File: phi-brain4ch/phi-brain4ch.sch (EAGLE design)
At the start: 65 parts, among them IC1 STM32F427VGT6, IC2 6N138S-TA1, IC3 AT45DB161D-SU, U1 LM1117MPX-3.3/NOPB or AP2114H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, U2 PRTR5V0U2X, X2 04-JST-B4B-XH-A, X3 04-JST-B4B-XH-A, Y1 8MHz

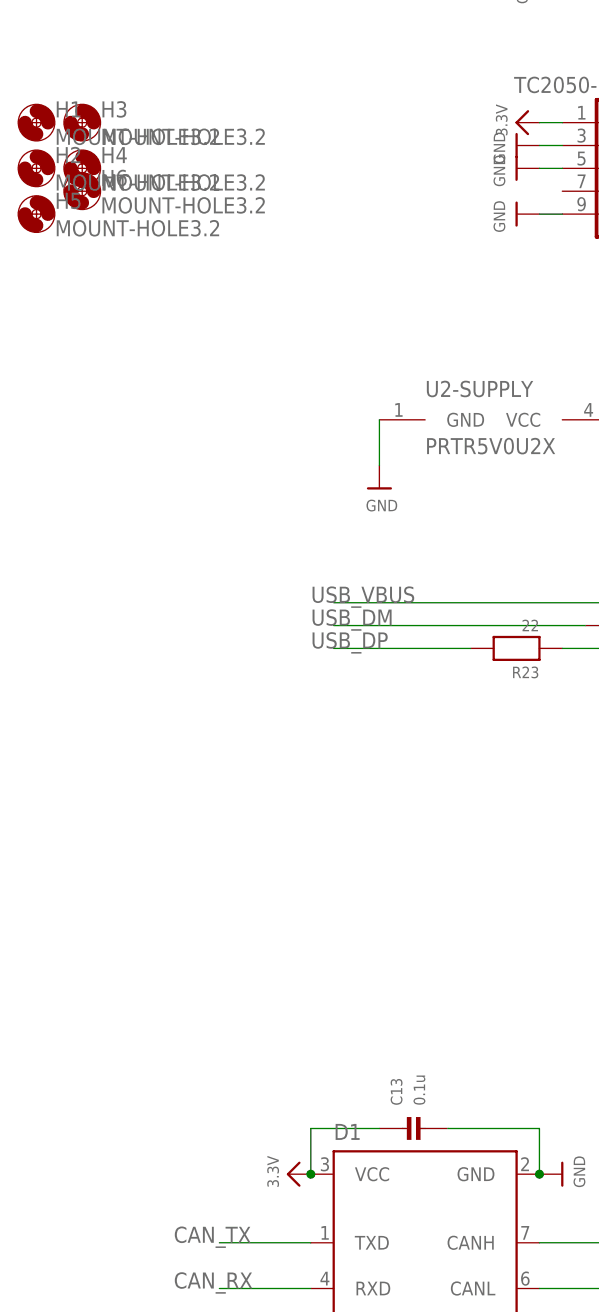
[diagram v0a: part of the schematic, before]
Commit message: wip
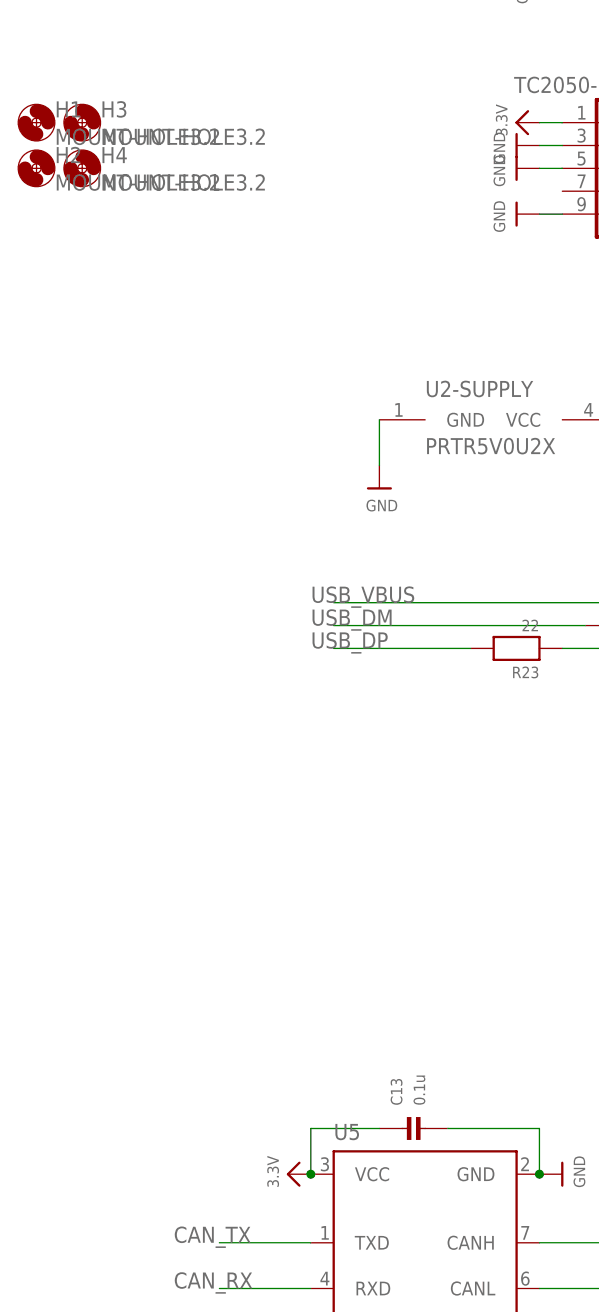
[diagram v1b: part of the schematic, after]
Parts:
- removed H5, H6: MOUNT-HOLE3.2, holes:MOUNT-HOLE3.2
- R5: device microbuilder:RESISTOR_0603 -> microbuilder:RESISTOR0805
- renumbered D1 to U5
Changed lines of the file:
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@@
 <part name="H1" library="holes" deviceset="MOUNT-HOLE" device="3.2"/>
 <part name="H2" library="holes" deviceset="MOUNT-HOLE" device="3.2"/>
-<part name="H5" library="holes" deviceset="MOUNT-HOLE" device="3.2"/>
-<part name="H6" library="holes" deviceset="MOUNT-HOLE" device="3.2"/>
 <part name="TC1" library="TagConnect" deviceset="TC2050-IDC" device="-NL"/>
 <part name="U$55" library="microbuilder" deviceset="3.3V" device=""/>
@@
 <part name="U2" library="Volks73-NXPSemiconductors" deviceset="PRTR5V0U2X?" device=""/>
 <part name="GND33" library="microbuilder" deviceset="GND" device=""/>
-<part name="D1" library="omc" deviceset="SN65HVD230" device="" value="SN65HVD230"/>
+<part name="U5" library="omc" deviceset="SN65HVD230" device="" value="SN65HVD230"/>
 <part name="GND12" library="microbuilder" deviceset="GND" device=""/>
 <part name="GND22" library="microbuilder" deviceset="GND" device=""/>
@@
 <part name="MIDI_OUT" library="keves" deviceset="MIDIJACK" device=""/>
 <part name="R4" library="microbuilder" deviceset="RESISTOR" device="0805" value="220"/>
-<part name="R5" library="microbuilder" deviceset="RESISTOR" device="_0603" value="220"/>
+<part name="R5" library="microbuilder" deviceset="RESISTOR" device="0805" value="220"/>
 <part name="R6" library="microbuilder" deviceset="RESISTOR" device="0805" value="220"/>
 <part name="IC2" library="6n138" deviceset="6N138" device="SMD" value="6N138S-TA1"/>
@@
 <instance part="H1" gate="G$1" x="-73.66" y="147.32"/>
 <instance part="H2" gate="G$1" x="-73.66" y="142.24"/>
-<instance part="H5" gate="G$1" x="-73.66" y="137.16"/>
-<instance part="H6" gate="G$1" x="-68.58" y="139.7"/>
 <instance part="TC1" gate="A" x="-7.62" y="142.24" rot="R180"/>
 <instance part="U$55" gate="G$1" x="-20.32" y="147.32" rot="R90"/>
@@
 <instance part="U2" gate="-SUPPLY" x="-22.86" y="114.3" rot="R270"/>
 <instance part="GND33" gate="G$1" x="-35.56" y="106.68"/>
-<instance part="D1" gate="G$1" x="-30.48" y="20.32"/>
+<instance part="U5" gate="G$1" x="-30.48" y="20.32"/>
 <instance part="GND12" gate="G$1" x="-48.26" y="10.16" rot="R270"/>
 <instance part="GND22" gate="G$1" x="-15.24" y="30.48" rot="R90"/>
@@
 </segment>
 <segment>
-<pinref part="D1" gate="G$1" pin="VCC"/>
+<pinref part="U5" gate="G$1" pin="VCC"/>
 <pinref part="3.3V8" gate="G$1" pin="3.3V"/>
 <pinref part="C13" gate="G$1" pin="P$1"/>
@@
 </segment>
 <segment>
-<pinref part="D1" gate="G$1" pin="GND"/>
+<pinref part="U5" gate="G$1" pin="GND"/>
 <pinref part="GND22" gate="G$1" pin="GND"/>
 <pinref part="C13" gate="G$1" pin="P$2"/>
@@
 </segment>
 <segment>
-<pinref part="D1" gate="G$1" pin="RS"/>
+<pinref part="U5" gate="G$1" pin="RS"/>
 <wire x1="-45.72" y1="10.16" x2="-43.18" y2="10.16" width="0.1524" layer="91"/>
 <pinref part="GND12" gate="G$1" pin="GND"/>
@@
 <net name="CAN_H" class="0">
 <segment>
-<pinref part="D1" gate="G$1" pin="CANH"/>
+<pinref part="U5" gate="G$1" pin="CANH"/>
 <wire x1="-17.78" y1="22.86" x2="-7.62" y2="22.86" width="0.1524" layer="91"/>
 <wire x1="-7.62" y1="22.86" x2="-7.62" y2="40.64" width="0.1524" layer="91"/>
@@
 <net name="CAN_L" class="0">
 <segment>
-<pinref part="D1" gate="G$1" pin="CANL"/>
+<pinref part="U5" gate="G$1" pin="CANL"/>
 <wire x1="-17.78" y1="17.78" x2="-10.16" y2="17.78" width="0.1524" layer="91"/>
 <wire x1="-10.16" y1="17.78" x2="-10.16" y2="2.54" width="0.1524" layer="91"/>
@@
 <segment>
 <label x="-58.42" y="22.86" size="1.778" layer="95"/>
-<pinref part="D1" gate="G$1" pin="TXD"/>
+<pinref part="U5" gate="G$1" pin="TXD"/>
 <wire x1="-53.34" y1="22.86" x2="-43.18" y2="22.86" width="0.1524" layer="91"/>
 </segment>
@@
 <segment>
 <label x="-58.42" y="17.78" size="1.778" layer="95"/>
-<pinref part="D1" gate="G$1" pin="RXD"/>
+<pinref part="U5" gate="G$1" pin="RXD"/>
 <wire x1="-43.18" y1="17.78" x2="-53.34" y2="17.78" width="0.1524" layer="91"/>
 </segment>
@@
 <net name="N$9" class="0">
 <segment>
-<pinref part="D1" gate="G$1" pin="VREF"/>
+<pinref part="U5" gate="G$1" pin="VREF"/>
 <wire x1="-17.78" y1="10.16" x2="15.24" y2="10.16" width="0.1524" layer="91"/>
 <wire x1="15.24" y1="10.16" x2="15.24" y2="15.24" width="0.1524" layer="91"/>

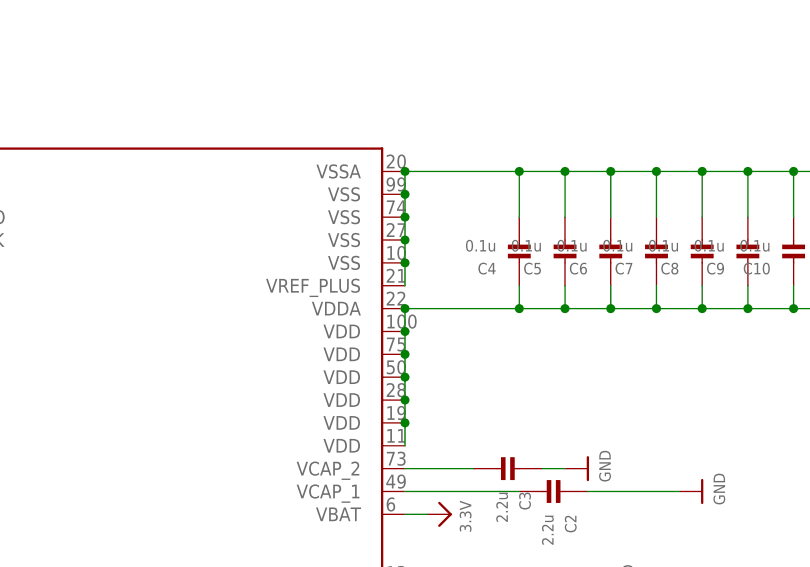
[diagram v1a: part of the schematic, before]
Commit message: wip
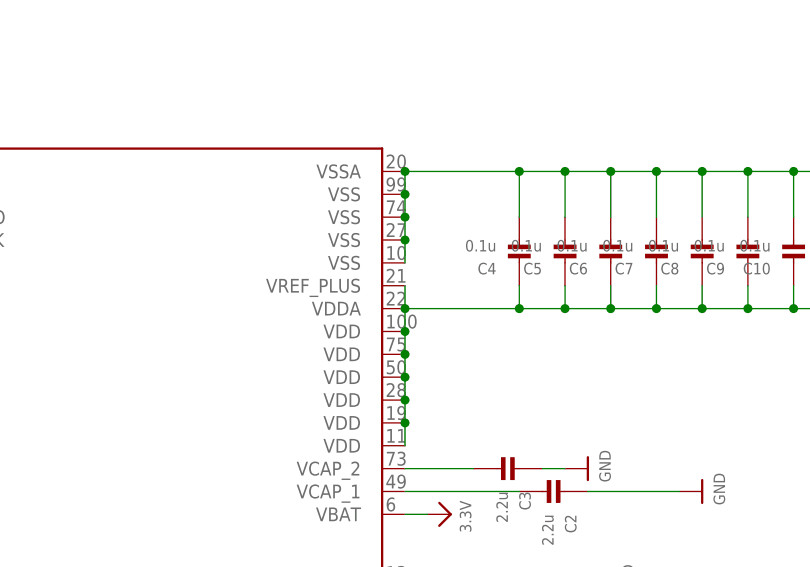
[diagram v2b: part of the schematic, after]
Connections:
- net 3.3V: now also IC1.VREF_PLUS
- net GND: no longer IC1.VREF_PLUS
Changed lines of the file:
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@@
 <junction x="147.32" y="127"/>
 <junction x="142.24" y="127"/>
+<pinref part="IC1" gate="G$1" pin="VREF_PLUS"/>
+<wire x1="129.54" y1="129.54" x2="129.54" y2="127" width="0.1524" layer="91"/>
 </segment>
 <segment>
@@
 <pinref part="IC1" gate="G$1" pin="VSS@1"/>
 <junction x="129.54" y="134.62"/>
-<pinref part="IC1" gate="G$1" pin="VREF_PLUS"/>
-<wire x1="129.54" y1="129.54" x2="129.54" y2="132.08" width="0.1524" layer="91"/>
-<junction x="129.54" y="132.08"/>
 <pinref part="C10" gate="G$1" pin="P$2"/>
 <wire x1="172.72" y1="137.16" x2="172.72" y2="142.24" width="0.1524" layer="91"/>
